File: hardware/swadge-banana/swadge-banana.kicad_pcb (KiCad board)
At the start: 2 copper layers, 80.5 x 127.3 mm, 46 parts, among them J1 USB_B_Micro, Q1 Q_NPN_BEC, SW1 SW_SPDT, U1 ESP-13-WROOM-02D, U3 BUS_PCIexpress, U4 QMA6981, U5 AP1117-33, U6 OLED_CONNECTOR

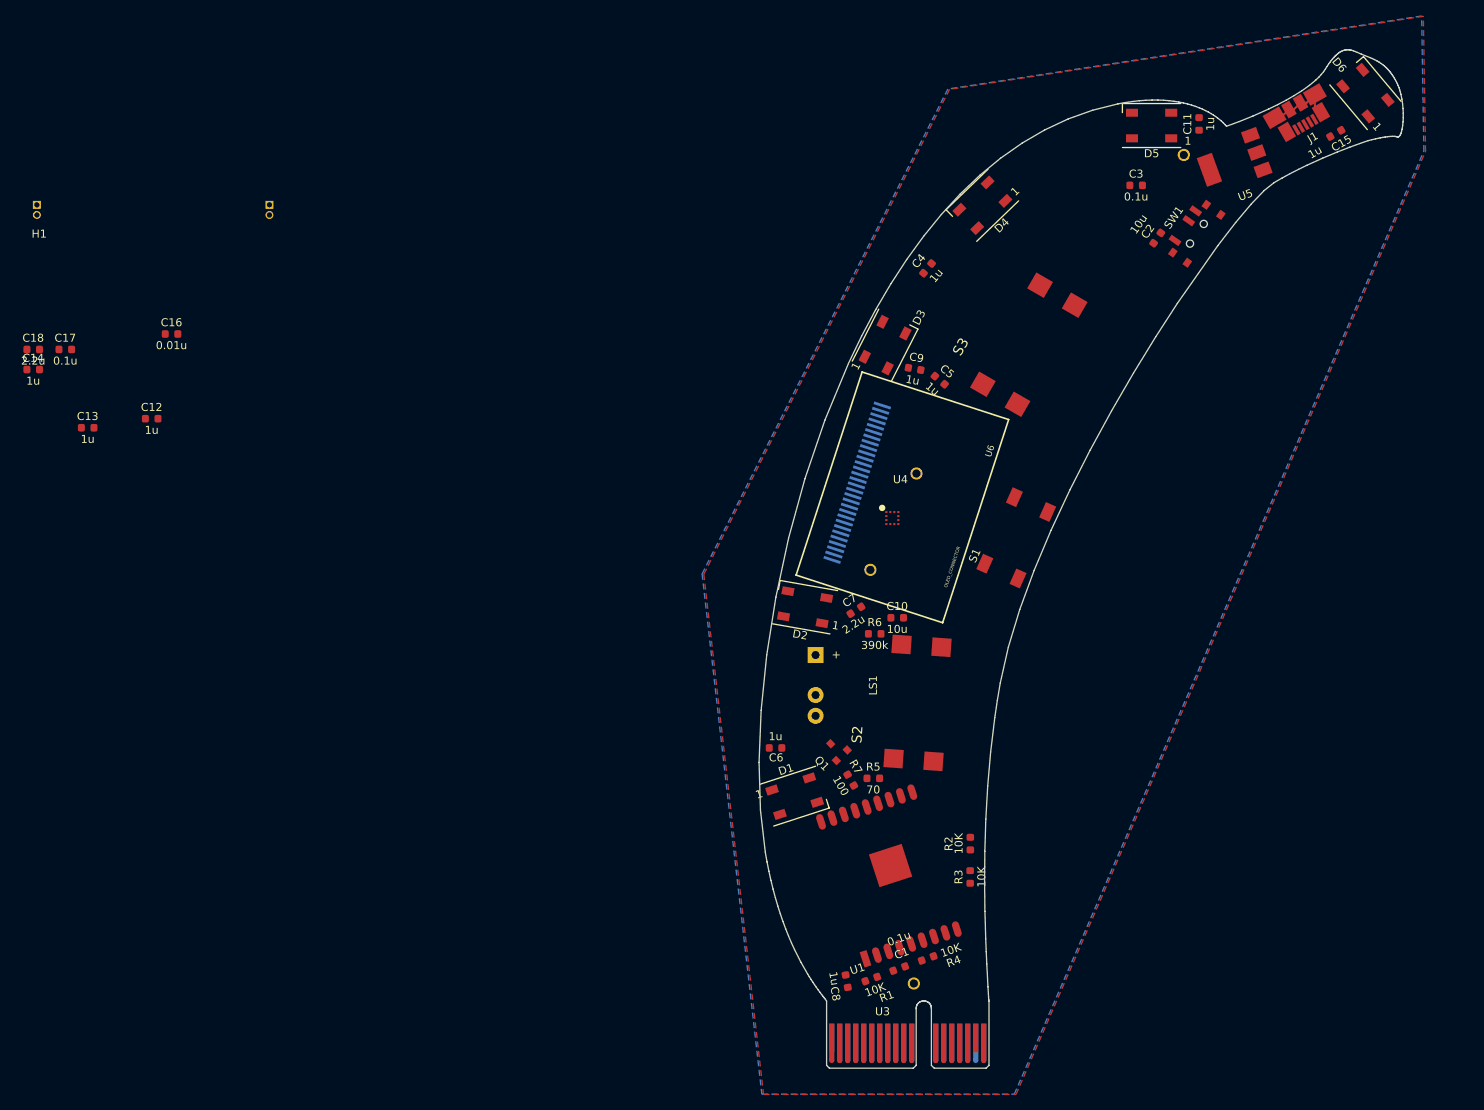
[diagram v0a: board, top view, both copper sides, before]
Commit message: Add my notional banana
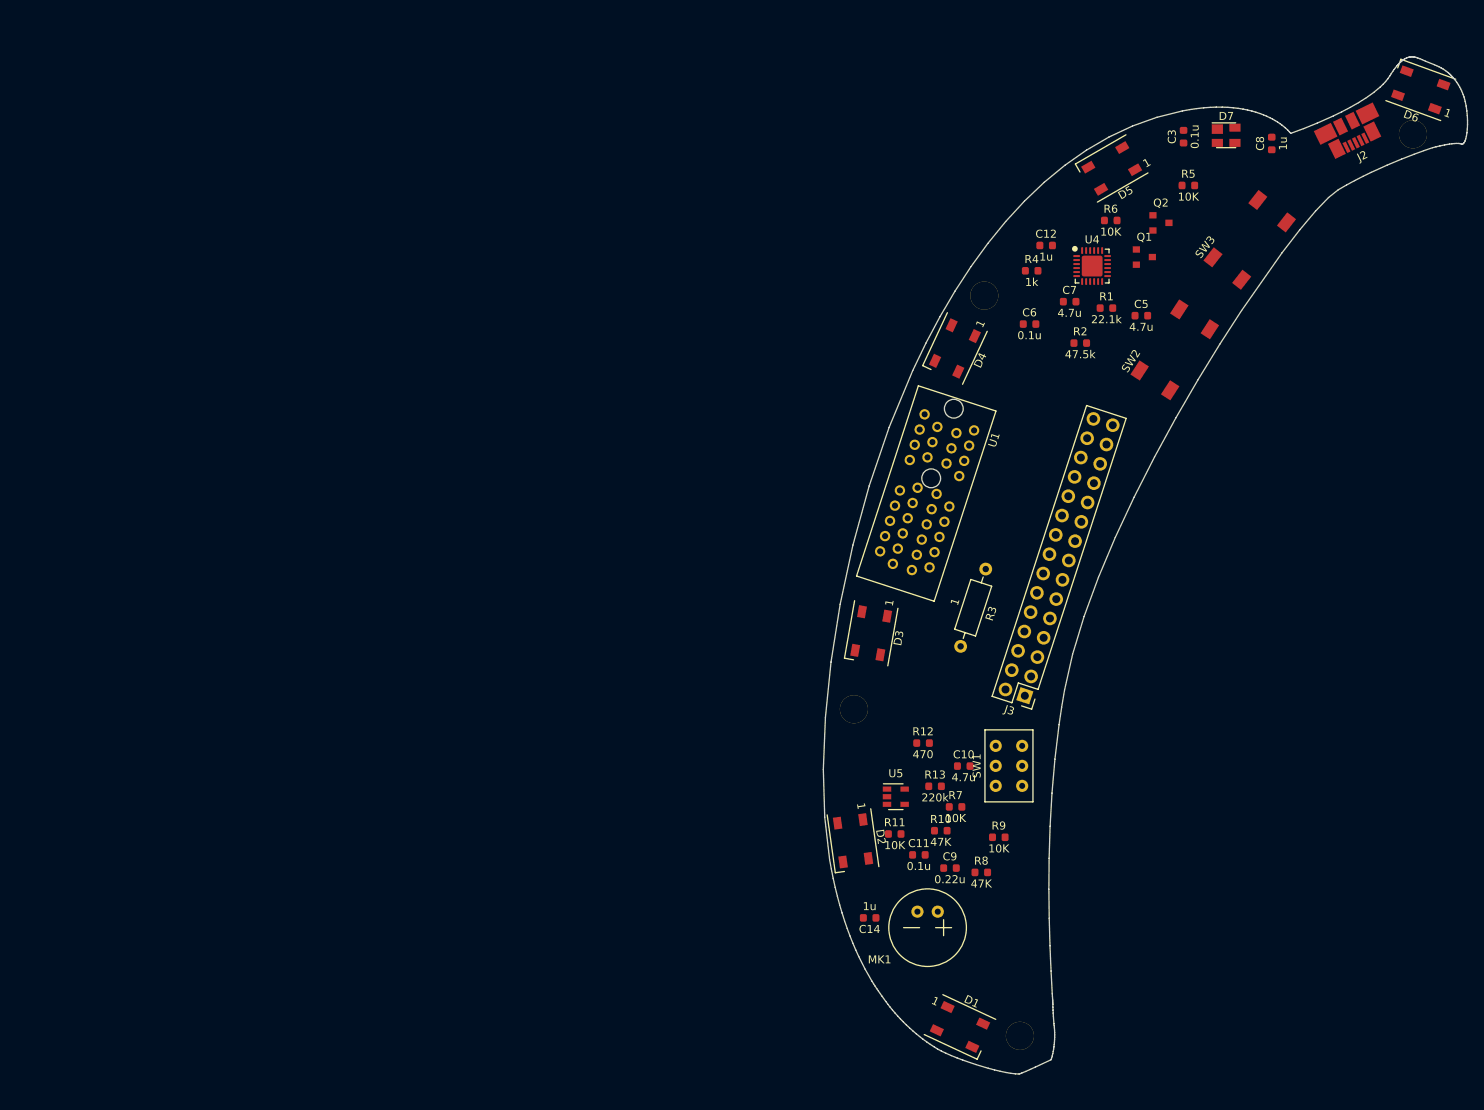
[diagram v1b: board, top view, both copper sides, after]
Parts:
- removed BT1, BT2: Battery, Swadge_Parts:2460
- removed C1, C17: 0.1u, Swadge_Parts:C_0603_1608Metric
- removed C13, C15, C4: 1u, Swadge_Parts:C_0603_1608Metric
- removed C16: 0.01u, Swadge_Parts:C_0603_1608Metric
- removed C18: 2.2u, Swadge_Parts:C_0603_1608Metric
- removed C2: 10u, Swadge_Parts:C_0603_1608Metric
- removed J1: USB_B_Micro, Swadge_Parts:USB_Micro-B_Molex_47346-0001
- removed LS1: Speaker, Swadge_Parts:Buzzer_12x9.5RM7.6
- removed S1: 4-1437565-2, Swadge_Parts:SW_4-1437565-2
- removed S2, S3: B3FS-4002P, Swadge_Parts:B3FS4002P
- removed U3: BUS_PCIexpress, Swadge_Parts:BUS_PCIexpress
- removed U6: OLED_CONNECTOR, Swadge_Parts:microbuilder-UG-2864HSWEG01_0.96IN_WRAPAROUND
- added D7: SP0503BAHT, Swadge_Parts:SOT-143, F.Cu at (168.9, 45.0)
- added H2: Hole, Swadge_Parts:Hole, F.Cu at (122.4, 116.8)
- added H3: Hole, Swadge_Parts:Hole, F.Cu at (138.7, 65.0)
- added H4: Hole, Swadge_Parts:Hole, F.Cu at (143.1, 157.6)
- added J2: USB_B_Micro, Swadge_Parts:USB_Micro-B_Molex_47346-0001, F.Cu at (184.5, 44.6)
- added J3: Conn_02x15_Top_Bottom, Swadge_Parts:PinHeader_2x15_P2.54mm_Vertical, F.Cu at (143.7, 115.1)
- added MK1: Microphone, Swadge_Parts:CMA-4544PF-W, F.Cu at (131.6, 144.1)
- added Q2: Q_NPN_BEC, Swadge_Parts:SOT-23, F.Cu at (160.8, 56.0)
- added R10: 47K, Swadge_Parts:R_0603_1608Metric, F.Cu at (133.2, 131.9)
- added R11: 10K, Swadge_Parts:R_0603_1608Metric, F.Cu at (127.5, 132.3)
- added R12: 470, Swadge_Parts:R_0603_1608Metric, F.Cu at (131.0, 121.0)
- added R13: 220k, Swadge_Parts:R_0603_1608Metric, F.Cu at (132.5, 126.4)
- added R8: 47K, Swadge_Parts:R_0603_1608Metric, F.Cu at (138.3, 137.1)
- added R9: 10K, Swadge_Parts:R_0603_1608Metric, F.Cu at (140.5, 132.8)
- added SW2: 4-1437565-2, Swadge_Parts:SW_4-1437565-2, F.Cu at (162.5, 71.8)
- added SW3: 4-1437565-2, Swadge_Parts:SW_4-1437565-2, F.Cu at (171.8, 58.1)
- C10: value 10u -> 4.7u
- C11, C6: value 1u -> 0.1u
- C5: value 1u -> 4.7u
- C7: value 2.2u -> 4.7u
- C9: value 1u -> 0.22u
- H1: value Headband -> Hole; footprint Swadge_Parts:Headband -> Swadge_Parts:Hole
- R1: value 10K -> 22.1k
- R2: value 10K -> 47.5k
- R3: value 10K -> 1; footprint Swadge_Parts:R_0603_1608Metric -> Swadge_Parts:R_Axial_DIN0207_L6.3mm_D2.5mm_P10.16mm_Horizontal
- R4: value 10K -> 1k
- R5: value 70 -> 10K
- R6: value 390k -> 10K
- R7: value 100 -> 10K
- SW1: value SW_SPDT -> SW_DPDT_x2; footprint Swadge_Parts:SW_SPDT_PCM12 -> Swadge_Parts:JS202011CQN
- U1: value ESP-13-WROOM-02D -> BUS_PCIexpress; footprint Swadge_Parts:ESP-13-WROOM-02 -> Swadge_Parts:10018784-10210TLF
- U4: value QMA6981 -> CP2102N-A01-GQFN24; footprint Swadge_Parts:QMA6981 -> Swadge_Parts:QFN-24-1EP_4x4mm_P0.5mm_EP2.6x2.6mm
- U5: value AP1117-33 -> MCP6001UT-I_OT; footprint Swadge_Parts:SOT-223-3_TabPin2 -> Swadge_Parts:SOT-23-5
- moved H1 157.8 mm to (192.2, 44.9)
- moved C14 125.0 mm to (124.3, 142.8), turned to 180 degrees
- moved C8 117.4 mm to (174.6, 46.0), turned to 90 degrees
- moved C12 113.9 mm to (146.4, 58.8)
- moved C11 97.9 mm to (130.5, 134.9), turned to 0 degrees
- moved U5 89.9 mm to (127.6, 127.7), turned to 0 degrees
- moved R1 88.9 mm to (153.9, 66.6), turned to 0 degrees
- moved R4 86.9 mm to (144.6, 61.9), turned to 0 degrees
- moved R5 83.9 mm to (164.2, 51.3)
- moved Q1 72.6 mm to (158.7, 60.2), turned to 0 degrees
- moved SW1 70.6 mm to (141.8, 123.8), turned to 90 degrees
- moved R2 64.1 mm to (150.7, 71.0), turned to 0 degrees
- moved C9 62.6 mm to (134.4, 136.6), turned to 0 degrees
- moved C6 61.8 mm to (144.3, 68.6), turned to 0 degrees
- moved U1 60.6 mm to (132.0, 87.9), turned to 72 degrees
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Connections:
- C10 pad 1: GND -> AUD_VCC
- C10 pad 2: Net-(C10-Pad2) -> GND
- C11 pad 1: +3V3 -> GND
- C11 pad 2: GND -> AUD_VCC
- C3 pad 1: GND -> Net-(C3-Pad1)
- C3 pad 2: +3V3 -> GND
- C5 pad 1: Net-(C5-Pad1) -> Net-(C3-Pad1)
- C5 pad 2: Net-(C5-Pad2) -> GND
- C6 pad 1: GND -> +3V3
- C6 pad 2: +3V3 -> GND
- C7 pad 1: GND -> +3V3
- C7 pad 2: Net-(C7-Pad2) -> GND
- D1 pad 4: Net-(D1-Pad4) -> LED_OUT
- D6 pad 2: LED_OUT -> Net-(D6-Pad2)
- Q1 pad 2: GND -> DTR_GPIO0
- Q1 pad 3: Net-(LS1-Pad2) -> SCL
- R1 pad 1: +3V3 -> Net-(C3-Pad1)
- R1 pad 2: Net-(C1-Pad2) -> Net-(R1-Pad2)
- R2 pad 1: +3V3 -> Net-(R1-Pad2)
- R2 pad 2: SCL -> GND
- R3 pad 1: +3V3 -> Net-(R3-Pad1)
- R3 pad 2: SDA -> 5V
- R4 pad 1: GND -> Net-(R4-Pad1)
- R4 pad 2: _RES -> +3V3
- R5 pad 1: Net-(D1-Pad4) -> Net-(Q1-Pad1)
- R5 pad 2: RX -> RTS_EN
- R6 pad 1: GND -> Net-(Q2-Pad1)
- R6 pad 2: Net-(R6-Pad2) -> DTR_GPIO0
- R7 pad 1: Net-(Q1-Pad1) -> Net-(C9-Pad1)
- R7 pad 2: BZR -> AUD_VCC
- SW1 pad 1: Net-(BT2-Pad1) -> 5V
- SW1 pad 2: +3V3 -> +5V
- SW1 pad 4: GND -> 5V
- SW1 pad 5: GND -> +5V
- SW1 pad 6: GND -> Net-(SW1-Pad6)
- U4 pad 1: GND -> Net-(U4-Pad1)
- U4 pad 10: (no net) -> Net-(U4-Pad10)
- U4 pad 11: (no net) -> Net-(U4-Pad11)
- U4 pad 12: SCL -> Net-(U4-Pad12)
- U4 pad 2: SDA -> GND
- U4 pad 3: +3V3 -> Net-(D7-Pad3)
- U4 pad 4: GND -> Net-(D7-Pad4)
- U4 pad 5: (no net) -> +3V3
- U4 pad 6: (no net) -> +3V3
- U4 pad 7: +3V3 -> Net-(C3-Pad1)
- U4 pad 8: GND -> Net-(R1-Pad2)
- U4 pad 9: GND -> Net-(R4-Pad1)
- U5 pad 1: GND -> ADC_PIN
- U5 pad 2: Net-(SW1-Pad3) -> GND
- U5 pad 3: +5V -> Net-(R10-Pad2)
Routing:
- net GND: track 8.78 -> 0.00 mm
- removed copper zone on B.Cu, net GND
- removed copper zone on F.Cu, net GND
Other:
- board size 80.5 x 127.3 mm -> 80.5 x 127.1 mm
